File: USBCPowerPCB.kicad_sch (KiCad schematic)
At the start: 36 parts, among them J1 UJ31-CH-31N-SMT-TR, J10 GND_BANANA_OUT, J11 12V_BANANA_IN, J12 GND_BANANA_IN, J2 CC, J3 12V_OUT, J4 5V_ISOOUT, J5 5V_UNISOOUT, J6 12V_OUT_PIN, J7 5V_ISOOUT_PIN, J8 5V_UNISOOUT_PIN, J9 12V_BANANA_OUT, U1 TVS2200DRV

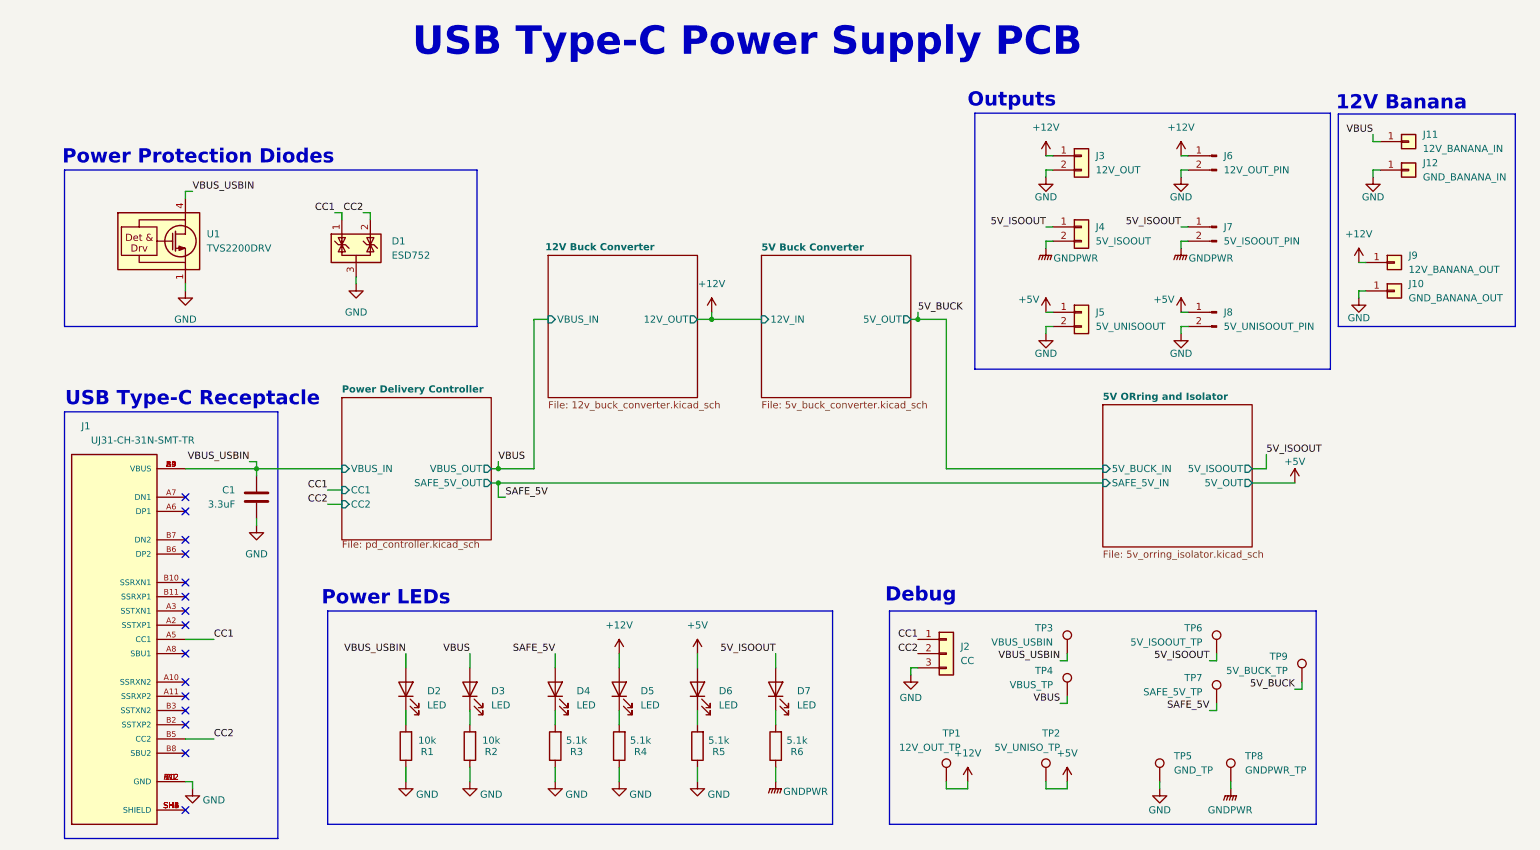
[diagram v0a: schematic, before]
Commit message: intermediate progress push before addressing Champers' and Lakshay's review comments
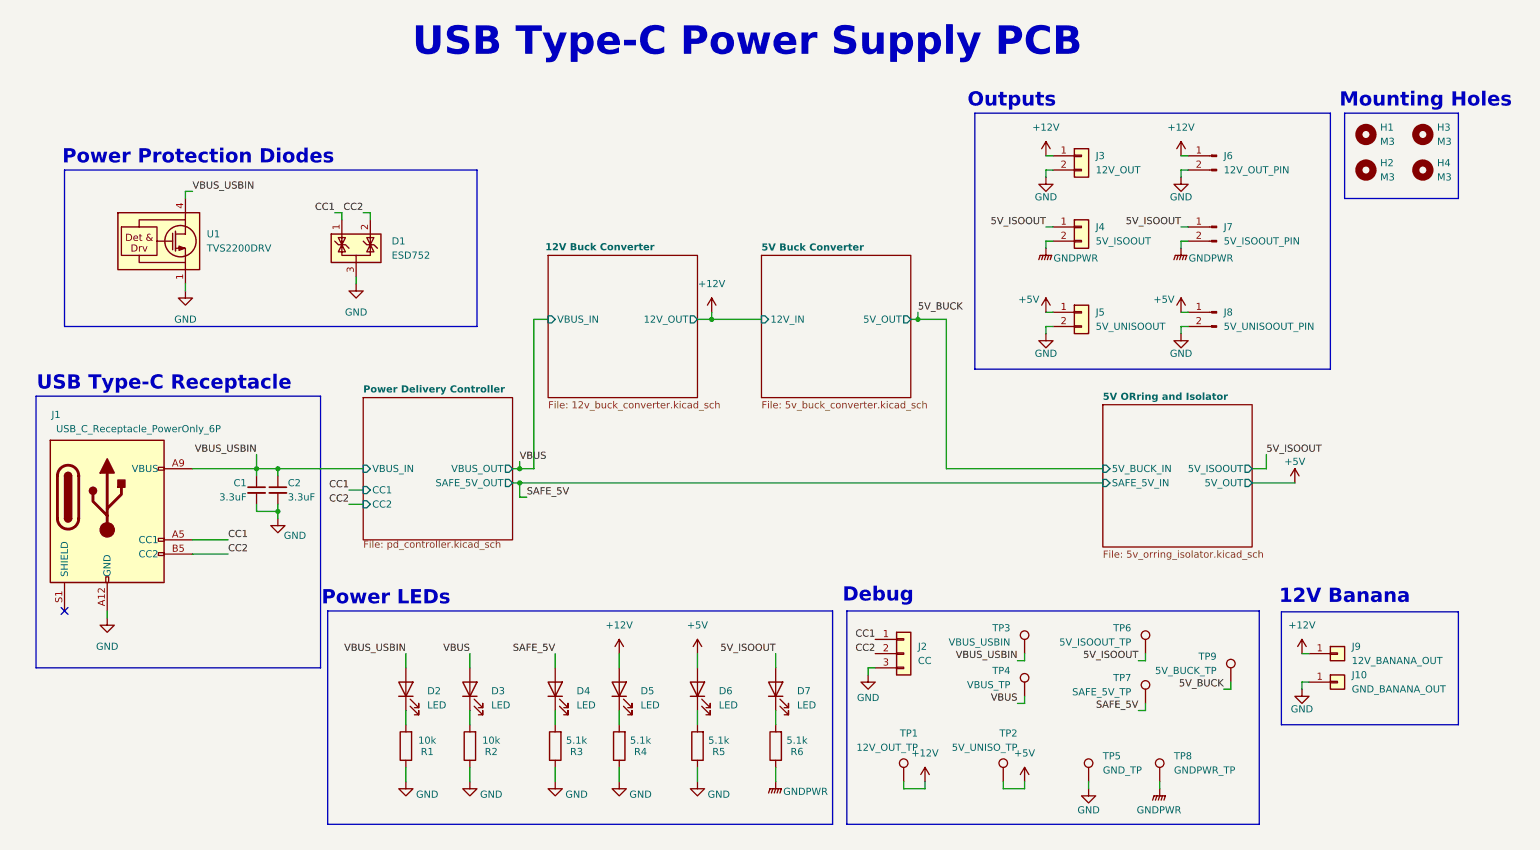
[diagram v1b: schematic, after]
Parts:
- removed J1: UJ31-CH-31N-SMT-TR, UTSVT_Connectors:CUI_UJ31-CH-31N-SMT-TR, symbol utsvt-connectors:UJ31-CH-31N-SMT-TR
- removed J11: 12V_BANANA_IN, UTSVT_Connectors:Banana_Jack_Horizontal, symbol Connector_Generic:Conn_01x01
- removed J12: GND_BANANA_IN, UTSVT_Connectors:Banana_Jack_Horizontal, symbol Connector_Generic:Conn_01x01
- added C2: 3.3uF, Capacitor_SMD:C_0805_2012Metric, symbol Device:C_Small
- added H1, H2, H3, H4: M3, MountingHole:MountingHole_3.2mm_M3, symbol Mechanical:MountingHole
- added J1: USB_C_Receptacle_PowerOnly_6P, UTSVT_Connectors:TYPEC31M17, symbol Connector:USB_C_Receptacle_PowerOnly_6P
- C1: symbol Device:C -> Device:C_Small
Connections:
- net CC1: now also J1.A5 (CC1)
- net CC2: now also J1.B5 (CC2)
- net GND: now also C2.2, J1.A12 (GND), J1.B12 (GND)
- net VBUS_USBIN: now also C2.1, J1.A9 (VBUS), J1.B9 (VBUS)
- no-connect marks 15 -> 1
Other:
- note added: "Mounting Holes"
- moved on the sheet: C1, J10, J2, J9, TP1, TP2, TP3, TP4, TP5, TP6, TP7, TP8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
